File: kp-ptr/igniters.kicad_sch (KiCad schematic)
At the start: 36 parts, among them J10 Conn_01x02, J11 Conn_01x02, J12 Conn_01x02, J13 Conn_01x02, Q2 DMC2025UFDB_v2, Q3 DMC2025UFDB_v2, Q4 DMC2025UFDB_v2, Q5 DMC2025UFDB_v2

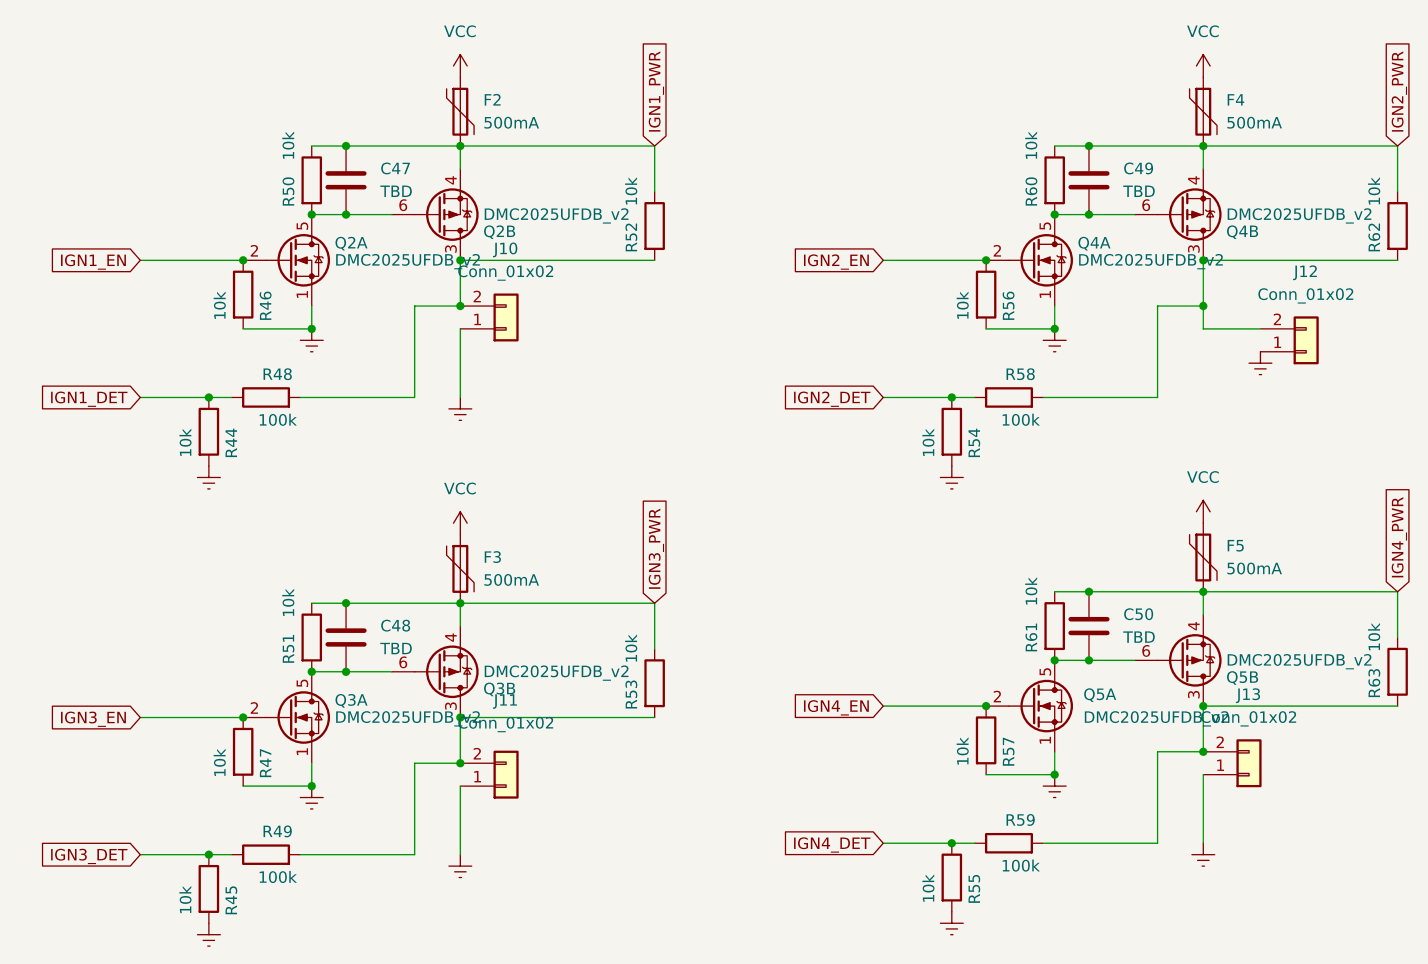
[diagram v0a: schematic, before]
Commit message: Update from v0.1 to v1.0
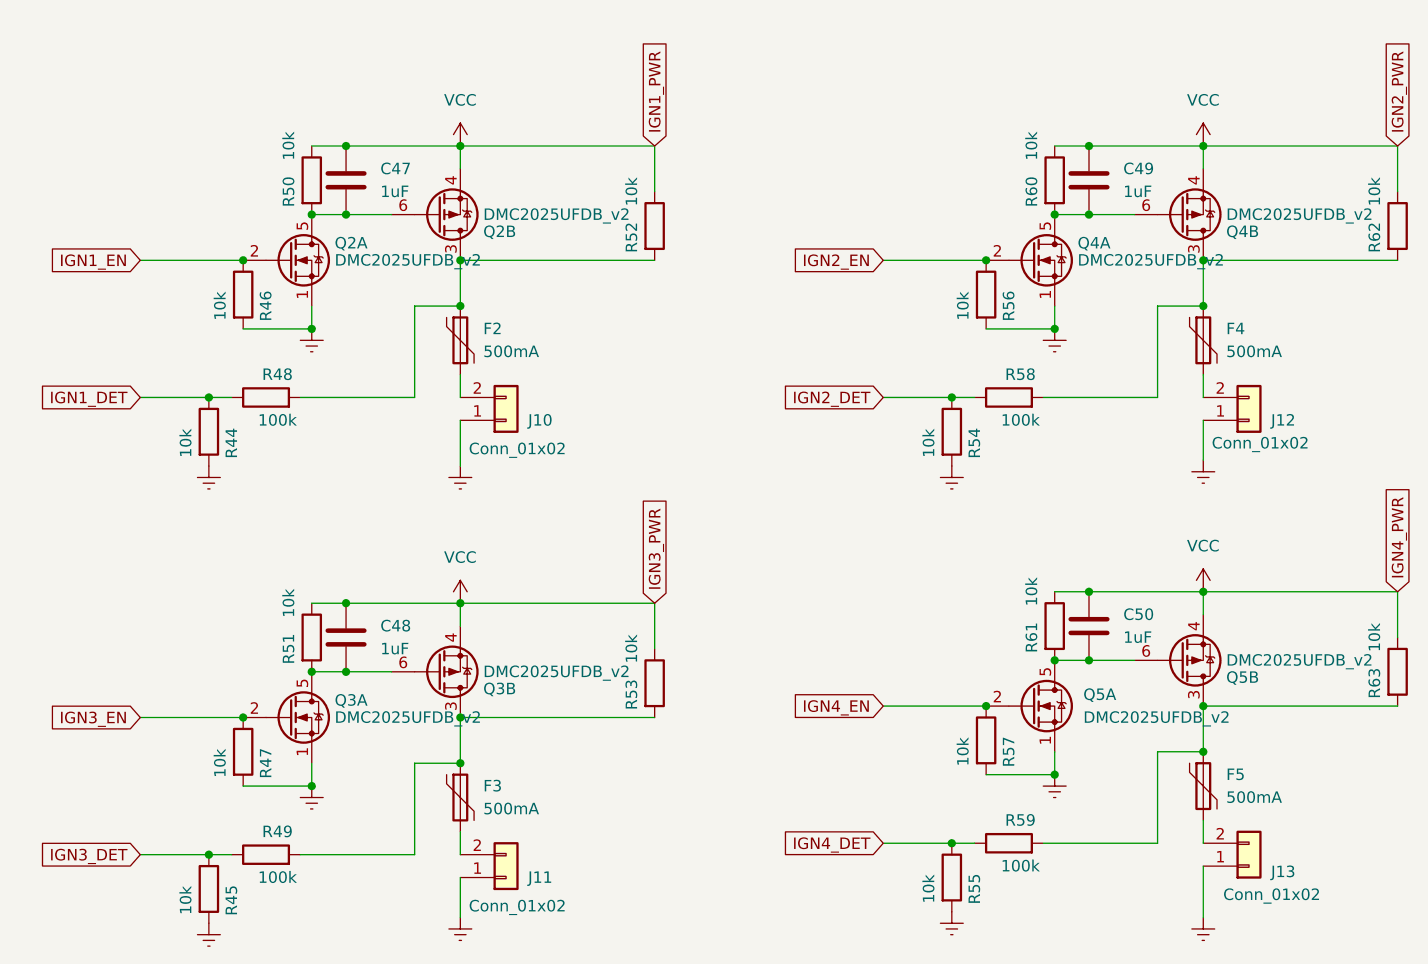
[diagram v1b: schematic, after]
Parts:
- C47, C48, C49, C50: value TBD -> 1uF
- F2, F3, F4, F5: footprint Fuse:Fuse_0805_2012Metric -> Fuse:Fuse_1210_3225Metric
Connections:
- net VCC: now also C47.1, C48.1, C49.1, C50.1, Q2.4 (S2), Q3.4 (S2), Q4.4 (S2), Q5.4 (S2), R50.1, R51.1, R52.1, R53.1, R60.1, R61.1, R62.1, R63.1; no longer F2.1, F3.1, F4.1, F5.1
- net at Q3.3 (D2), R49.2, R53.2: now also F3.1; no longer J11.2 (Pin_2)
- net at Q5.3 (D2), R59.2, R63.2: now also F5.1; no longer J13.2 (Pin_2)
- net at Q2.3 (D2), R48.2, R52.2: now also F2.1; no longer J10.2 (Pin_2)
- net at Q4.3 (D2), R58.2, R62.2: now also F4.1; no longer J12.2 (Pin_2)
- removed net IGN1_PWR: C47.1, F2.2, Q2.4 (S2), R50.1, R52.1
- removed net IGN2_PWR: C49.1, F4.2, Q4.4 (S2), R60.1, R62.1
- removed net IGN3_PWR: C48.1, F3.2, Q3.4 (S2), R51.1, R53.1
- removed net IGN4_PWR: C50.1, F5.2, Q5.4 (S2), R61.1, R63.1
- new net: F5.2, J13.2 (Pin_2)
- new net: F2.2, J10.2 (Pin_2)
- new net: F4.2, J12.2 (Pin_2)
- new net: F3.2, J11.2 (Pin_2)
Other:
- moved on the sheet: F2, F3, F4, F5, J10, J11, J12, J13

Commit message: Work in progress
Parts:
- F2, F3, F4, F5: footprint Fuse:Fuse_1210_3225Metric -> Fuse:Fuse_1206_3216Metric
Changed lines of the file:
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@@
       (effects (font (size 1.27 1.27)) (justify left))
     )
-    (property "Footprint" "Fuse:Fuse_1210_3225Metric" (id 2) (at 171.45 93.98 0)
+    (property "Footprint" "Fuse:Fuse_1206_3216Metric" (id 2) (at 171.45 93.98 0)
       (effects (font (size 1.27 1.27)) (justify left) hide)
     )
@@
       (effects (font (size 1.27 1.27)) (justify left))
     )
-    (property "Footprint" "Fuse:Fuse_1210_3225Metric" (id 2) (at 88.9 93.98 0)
+    (property "Footprint" "Fuse:Fuse_1206_3216Metric" (id 2) (at 88.9 93.98 0)
       (effects (font (size 1.27 1.27)) (justify left) hide)
     )
@@
       (effects (font (size 1.27 1.27)) (justify left))
     )
-    (property "Footprint" "Fuse:Fuse_1210_3225Metric" (id 2) (at 88.9 144.78 0)
+    (property "Footprint" "Fuse:Fuse_1206_3216Metric" (id 2) (at 88.9 144.78 0)
       (effects (font (size 1.27 1.27)) (justify left) hide)
     )
@@
       (effects (font (size 1.27 1.27)) (justify left))
     )
-    (property "Footprint" "Fuse:Fuse_1210_3225Metric" (id 2) (at 171.45 143.51 0)
-      (effects (font (size 1.27 1.27)) (justify left) hide)
-    )
+    (property "Footprint" "Fuse:Fuse_1206_3216Metric" (id 2) (at 171.45 143.51 0)
+      (effects (font (size 1.27 1.27)) (justify left) hide)
+    )
